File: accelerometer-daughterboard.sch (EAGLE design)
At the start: 4 parts, among them U1 LIS3DHTR

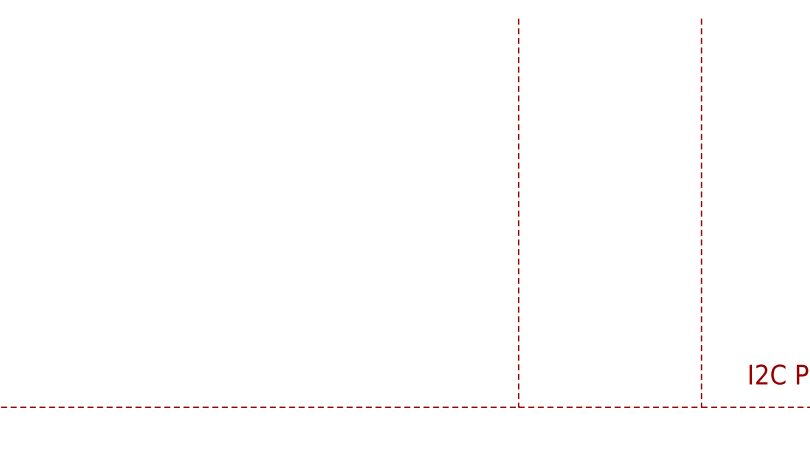
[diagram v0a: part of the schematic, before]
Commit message: Re-add buffer caps
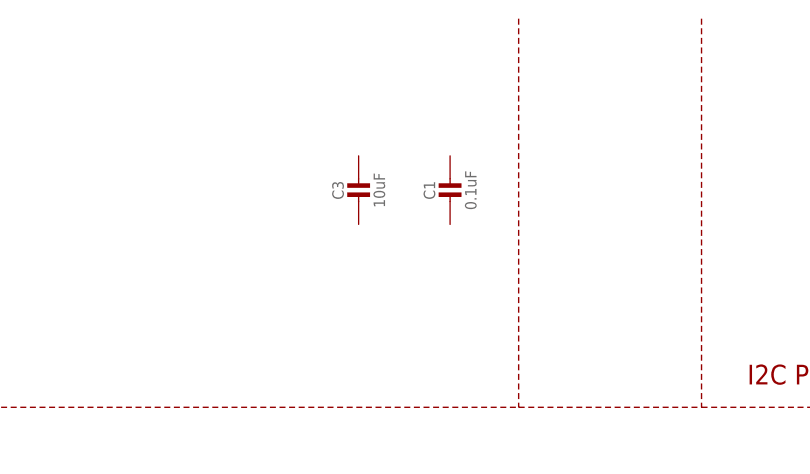
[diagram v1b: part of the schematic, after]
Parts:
- added C1: 0.1uF, microbuilder:CAP_CERAMIC0603_NO
- added C3: 10uF, microbuilder:CAP_CERAMIC0805-NOOUTLINE
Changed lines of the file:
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@@
 </classes>
 <parts>
+<part name="C3" library="microbuilder" deviceset="CAP_CERAMIC" device="0805-NOOUTLINE" value="10uF"/>
+<part name="C1" library="microbuilder" deviceset="CAP_CERAMIC" device="0603_NO" value="0.1uF"/>
 <part name="U$7" library="microbuilder" deviceset="3.3V" device=""/>
 <part name="U$24" library="microbuilder" deviceset="3.3V" device=""/>
@@
 <attribute name="SHEET" x="230.505" y="10.16" size="2.54" layer="94" font="vector"/>
 </instance>
+<instance part="C3" gate="G$1" x="50.8" y="154.94" smashed="yes">
+<attribute name="NAME" x="48.51" y="156.19" size="1.27" layer="95" font="vector" rot="R90" align="center"/>
+<attribute name="VALUE" x="53.1" y="156.19" size="1.27" layer="96" font="vector" rot="R90" align="center"/>
+</instance>
+<instance part="C1" gate="G$1" x="60.96" y="154.94" smashed="yes">
+<attribute name="NAME" x="58.67" y="156.19" size="1.27" layer="95" font="vector" rot="R90" align="center"/>
+<attribute name="VALUE" x="63.26" y="156.19" size="1.27" layer="96" font="vector" rot="R90" align="center"/>
+</instance>
 <instance part="U$7" gate="G$1" x="165.1" y="170.18" smashed="yes" rot="MR0">

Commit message: remove caps again
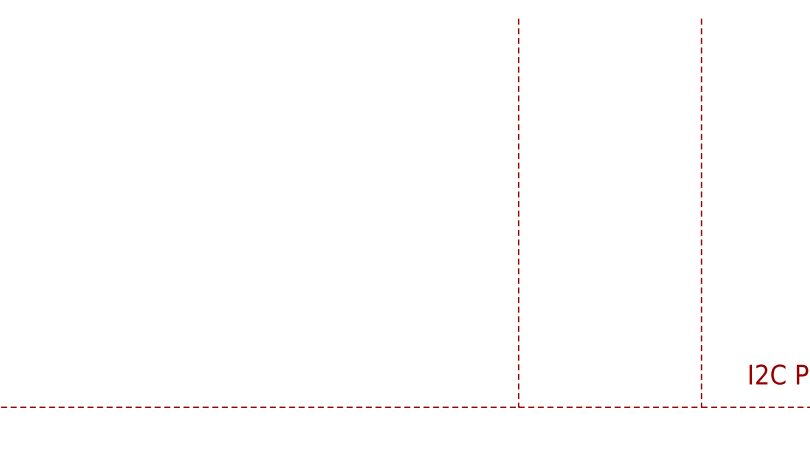
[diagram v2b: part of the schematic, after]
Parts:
- removed C1: 0.1uF, microbuilder:CAP_CERAMIC0603_NO
- removed C3: 10uF, microbuilder:CAP_CERAMIC0805-NOOUTLINE
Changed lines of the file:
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@@
 </classes>
 <parts>
-<part name="C3" library="microbuilder" deviceset="CAP_CERAMIC" device="0805-NOOUTLINE" value="10uF"/>
-<part name="C1" library="microbuilder" deviceset="CAP_CERAMIC" device="0603_NO" value="0.1uF"/>
 <part name="U$7" library="microbuilder" deviceset="3.3V" device=""/>
 <part name="U$24" library="microbuilder" deviceset="3.3V" device=""/>
@@
 <attribute name="SHEET" x="230.505" y="10.16" size="2.54" layer="94" font="vector"/>
 </instance>
-<instance part="C3" gate="G$1" x="50.8" y="154.94" smashed="yes">
-<attribute name="NAME" x="48.51" y="156.19" size="1.27" layer="95" font="vector" rot="R90" align="center"/>
-<attribute name="VALUE" x="53.1" y="156.19" size="1.27" layer="96" font="vector" rot="R90" align="center"/>
-</instance>
-<instance part="C1" gate="G$1" x="60.96" y="154.94" smashed="yes">
-<attribute name="NAME" x="58.67" y="156.19" size="1.27" layer="95" font="vector" rot="R90" align="center"/>
-<attribute name="VALUE" x="63.26" y="156.19" size="1.27" layer="96" font="vector" rot="R90" align="center"/>
-</instance>
 <instance part="U$7" gate="G$1" x="165.1" y="170.18" smashed="yes" rot="MR0">
